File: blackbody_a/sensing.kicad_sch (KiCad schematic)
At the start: 4 parts, among them U1 LTC4311CSC6-TRPBF

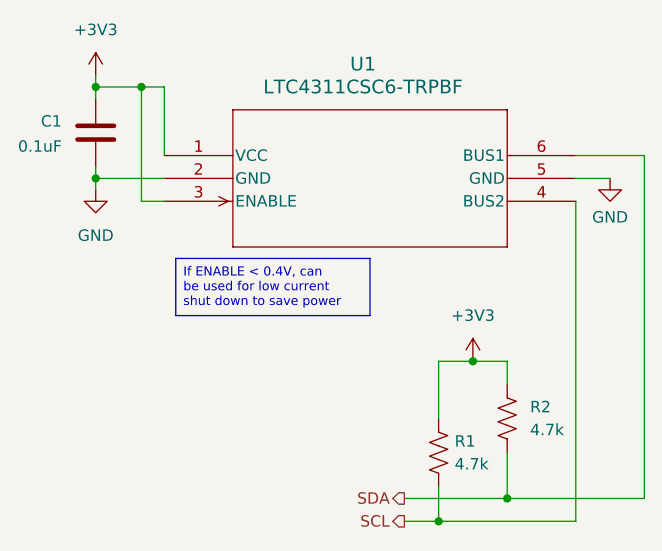
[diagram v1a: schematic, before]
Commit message: layout iteration 1
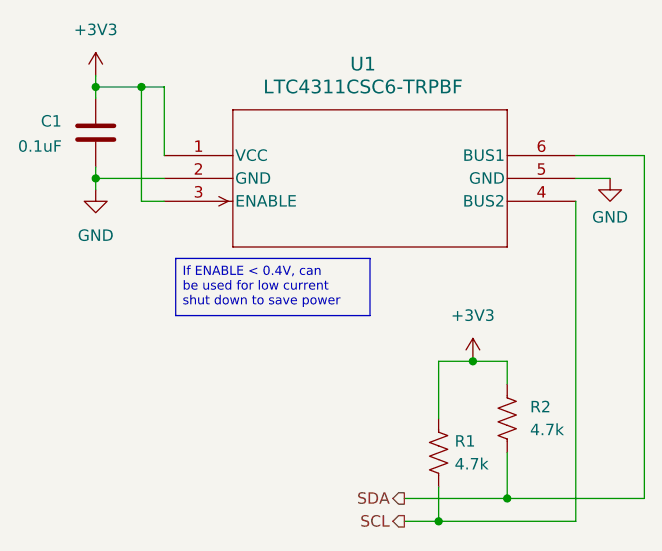
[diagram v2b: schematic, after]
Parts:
- C1: footprint (none) -> Capacitor_SMD:C_0805_2012Metric
- R1, R2: footprint (none) -> Resistor_SMD:R_0805_2012Metric
- U1: footprint SOT-6_SC_LIT -> blackbody_a:SOT-6_SC_LIT
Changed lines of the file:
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@@
 (kicad_sch
-	(version 20231120)
+	(version 20250114)
 	(generator "eeschema")
-	(generator_version "8.0")
+	(generator_version "9.0")
 	(paper "A4")
+	(text_box "If ENABLE < 0.4V, can be used for low current shut down to save power"
+		(exclude_from_sim no)
+		(at 85.09 71.12 0)
+		(size 21.59 6.35)
+		(margins 0.762 0.762 0.762 0.762)
+		(stroke
+			(width 0)
+			(type default)
+		)
+		(fill
+			(type none)
+		)
+		(effects
+			(font
+				(size 1.016 1.016)
+			)
+			(justify left top)
+		)
+	)
 	(junction
 		(at 81.28 52.07)
@@
 		)
 	)
-	(text_box "If ENABLE < 0.4V, can be used for low current shut down to save power"
-		(exclude_from_sim no)
-		(at 85.09 71.12 0)
-		(size 21.59 6.35)
-		(stroke
-			(width 0)
-			(type default)
-		)
-		(fill
-			(type none)
-		)
-		(effects
-			(font
-				(size 1.016 1.016)
-			)
-			(justify left top)
-		)
-	)
 	(hierarchical_label "SCL"
 		(shape output)
 		(at 110.49 100.33 180)
-		(fields_autoplaced yes)
 		(effects
 			(font
@@
 		(shape output)
 		(at 110.49 97.79 180)
-		(fields_autoplaced yes)
 		(effects
 			(font
@@
 			)
 		)
-		(property "Footprint" ""
+		(property "Footprint" "Resistor_SMD:R_0805_2012Metric"
 			(at 115.316 92.964 90)
 			(effects
@@
 			)
 		)
-		(property "Footprint" "SOT-6_SC_LIT"
+		(property "Footprint" "blackbody_a:SOT-6_SC_LIT"
 			(at 83.82 59.69 0)
 			(effects
@@
 			)
 		)
-		(property "Footprint" ""
+		(property "Footprint" "Resistor_SMD:R_0805_2012Metric"
 			(at 122.936 89.154 90)
 			(effects
@@
 			)
 		)
-		(property "Footprint" ""
+		(property "Footprint" "Capacitor_SMD:C_0805_2012Metric"
 			(at 75.2348 53.34 0)
 			(effects
